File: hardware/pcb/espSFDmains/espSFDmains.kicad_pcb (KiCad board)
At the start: 4 copper layers, 111.8 x 63.5 mm, 40 parts, among them J1 Mains, J10 D1 & D2, J11 D3 & D4, J2 Mains Motor, J3 VDD, J4 D5 & D6, J5 Motor, J8 SFD Bus, J9 SFD Bus, U1 TXS0102DCT, U2 LM2675N-5, U3 WEMOS_D1_mini

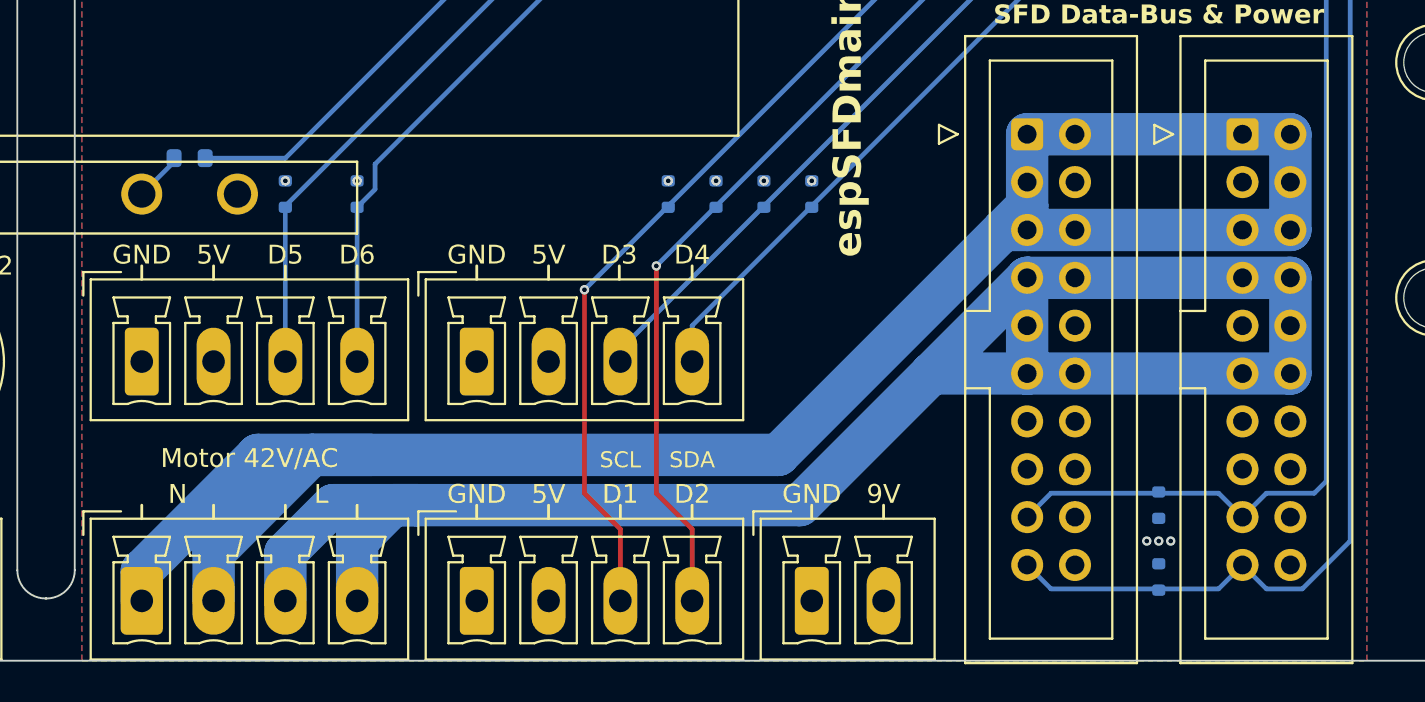
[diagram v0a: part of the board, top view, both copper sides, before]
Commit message: hedfhf
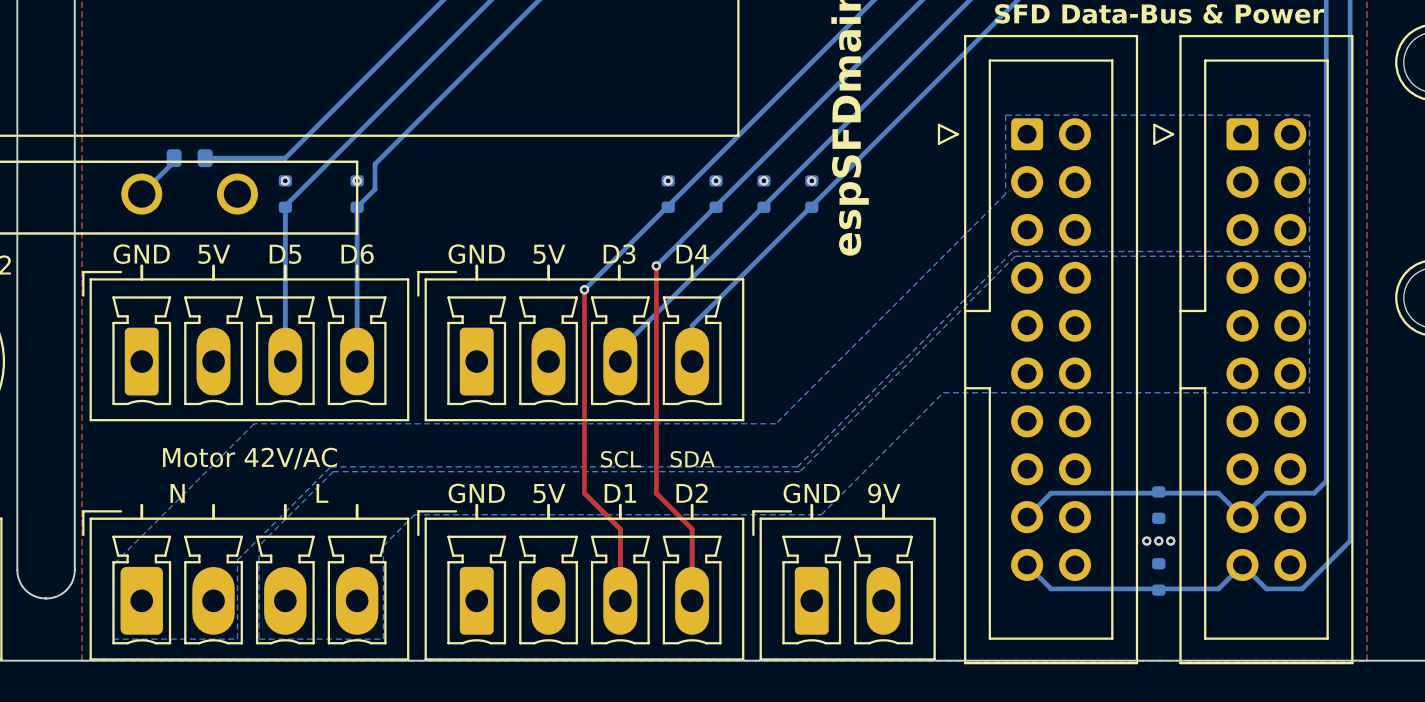
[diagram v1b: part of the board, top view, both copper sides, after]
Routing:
- net Motor N: track 109.0 -> 0.00 mm
- net Motor L: track 100.2 -> 0.00 mm
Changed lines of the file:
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@@
-	)
-	(segment
-		(start 117.155 140.01)
-		(end 122.235 134.93)
-		(width 2.25)
-		(layer "B.Cu")
-		(net 1)
-	)
-	(segment
-		(start 89.85 146.995)
-		(end 88.58 146.995)
-		(width 2.25)
-		(layer "B.Cu")
-		(net 1)
-	)
-	(segment
-		(start 86.675 148.9)
-		(end 86.675 152.075)
-		(width 2.25)
-		(layer "B.Cu")
-		(net 1)
-	)
-	(segment
-		(start 86.675 148.9)
-		(end 86.675 146.995)
-		(width 2.25)
-		(layer "B.Cu")
-		(net 1)
-	)
-	(segment
-		(start 89.85 146.995)
-		(end 86.675 146.995)
-		(width 2.25)
-		(layer "B.Cu")
-		(net 1)
-	)
-	(segment
-		(start 122.235 134.93)
-		(end 122.235 140.01)
-		(width 2.25)
-		(layer "B.Cu")
-		(net 1)
-	)
-	(segment
-		(start 110.17 146.995)
-		(end 117.155 140.01)
-		(width 2.25)
-		(layer "B.Cu")
-		(net 1)
-	)
-	(segment
-		(start 136.205 140.01)
-		(end 122.235 140.01)
-		(width 2.25)
-		(layer "B.Cu")
-		(net 1)
-	)
-	(segment
-		(start 122.235 140.01)
-		(end 117.155 140.01)
-		(width 2.25)
-		(layer "B.Cu")
-		(net 1)
-	)
-	(segment
-		(start 122.235 134.93)
-		(end 136.205 134.93)
-		(width 2.25)
-		(layer "B.Cu")
-		(net 1)
-	)
-	(segment
-		(start 82.865 149.535)
-		(end 82.865 152.075)
-		(width 2.25)
-		(layer "B.Cu")
-		(net 1)
-	)
-	(segment
-		(start 89.85 146.995)
-		(end 110.17 146.995)
-		(width 2.25)
-		(layer "B.Cu")
-		(net 1)
-	)
-	(segment
-		(start 88.58 146.995)
-		(end 86.675 148.9)
-		(width 2.25)
-		(layer "B.Cu")
-		(net 1)
-	)
-	(segment
-		(start 86.675 146.995)
-		(end 85.405 146.995)
-		(width 2.25)
-		(layer "B.Cu")
-		(net 1)
-	)
-	(segment
-		(start 136.205 134.93)
-		(end 136.205 140.01)
-		(width 2.25)
-		(layer "B.Cu")
-		(net 1)
-	)
-	(segment
-		(start 85.405 146.995)
-		(end 82.865 149.535)
-		(width 2.25)
-		(layer "B.Cu")
-		(net 1)
-	)
-	(segment
-		(start 79.055 149.535)
-		(end 84.262 144.328)
-		(width 2.25)
-		(layer "B.Cu")
-		(net 2)
-	)
-	(segment
-		(start 122.235 131.12)
-		(end 122.235 127.31)
-		(width 2.25)
-		(layer "B.Cu")
-		(net 2)
-	)
-	(segment
-		(start 75.245 150.4875)
-		(end 75.245 152.075)
-		(width 2.25)
-		(layer "B.Cu")
-		(net 2)
-	)
-	(segment
-		(start 79.055 152.075)
-		(end 79.055 149.535)
-		(width 2.25)
-		(layer "B.Cu")
-		(net 2)
-	)
-	(segment
-		(start 120.965 132.39)
-		(end 122.235 131.12)
-		(width 2.25)
-		(layer "B.Cu")
-		(net 2)
-	)
-	(segment
-		(start 122.235 127.31)
-		(end 136.205 127.31)
-		(width 2.25)
-		(layer "B.Cu")
-		(net 2)
-	)
-	(segment
-		(start 109.027 144.328)
-		(end 120.965 132.39)
-		(width 2.25)
-		(layer "B.Cu")
-		(net 2)
-	)
-	(segment
-		(start 136.205 132.39)
-		(end 122.235 132.39)
-		(width 2.25)
-		(layer "B.Cu")
-		(net 2)
-	)
-	(segment
-		(start 81.4045 144.328)
-		(end 75.245 150.4875)
-		(width 2.25)
-		(layer "B.Cu")
-		(net 2)
-	)
-	(segment
-		(start 136.205 127.31)
-		(end 136.205 132.39)
-		(width 2.25)
-		(layer "B.Cu")
-		(net 2)
-	)
-	(segment
-		(start 122.235 132.39)
-		(end 122.235 131.12)
-		(width 2.25)
-		(layer "B.Cu")
-		(net 2)
-	)
-	(segment
-		(start 84.262 144.328)
-		(end 109.027 144.328)
-		(width 2.25)
-		(layer "B.Cu")
-		(net 2)
-	)
-	(segment
-		(start 120.965 132.39)
-		(end 122.235 132.39)
-		(width 2.25)
-		(layer "B.Cu")
-		(net 2)
-	)
-	(segment
-		(start 87.437 144.328)
-		(end 81.4045 144.328)
-		(width 2.25)
-		(layer "B.Cu")
-		(net 2)
 	)
 	(segment
@@
 	)
 	(zone
-		(net 2)
-		(net_name "Motor N")
-		(layer "B.Cu")
-		(hatch edge 0.5)
-		(priority 4)
-		(connect_pads yes
-			(clearance 0.2)
-		)
-		(min_thickness 0.25)
-		(filled_areas_thickness no)
-		(fill yes
-			(thermal_gap 0.5)
-			(thermal_bridge_width 0.5)
-		)
-		(polygon
-			(pts
-				(xy 122.235 127.31) (xy 122.235 132.39) (xy 136.205 132.39) (xy 136.205 127.31)
-			)
-		)
-	)
-	(zone
 		(net 10)
 		(net_name "+9V")
@@
 		(layer "B.Cu")
 		(hatch edge 0.5)
-		(priority 4)
-		(connect_pads yes
-			(clearance 0.2)
-		)
-		(min_thickness 0.25)
-		(filled_areas_thickness no)
-		(fill yes
-			(thermal_gap 0.5)
-			(thermal_bridge_width 0.5)
-		)
-		(polygon
-			(pts
-				(xy 122.235 134.93) (xy 136.205 134.93) (xy 136.205 140.01) (xy 117.155 140.01)
-			)
-		)
-	)
-	(zone
-		(net 31)
-		(net_name "+5V")
-		(layer "B.Cu")
-		(hatch edge 0.5)
-		(priority 1)
+		(priority 7)
 		(connect_pads yes
 			(clearance 0.2)
@@
 		(polygon
 			(pts
+				(xy 137.221 133.787) (xy 121.6 133.787) (xy 110.17 145.217) (xy 85.405 145.217) (xy 81.468 149.154)
+				(xy 81.468 154.107) (xy 88.072 154.107) (xy 88.072 149.154) (xy 89.723 147.503) (xy 111.313 147.503)
+				(xy 117.79 141.026) (xy 137.221 141.026)
+			)
+		)
+	)
+	(zone
+		(net 31)
+		(net_name "+5V")
+		(layer "B.Cu")
+		(hatch edge 0.5)
+		(priority 1)
+		(connect_pads yes
+			(clearance 0.2)
+		)
+		(min_thickness 0.25)
+		(filled_areas_thickness no)
+		(fill yes
+			(thermal_gap 0.5)
+			(thermal_bridge_width 0.5)
+			(smoothing fillet)
+			(radius 0.25)
+		)
+		(polygon
+			(pts
 				(xy 87.818 109.911) (xy 84.135 109.911) (xy 80.071 105.847) (xy 80.071 99.751) (xy 83.119 96.83)
 				(xy 83.119 95.687) (xy 83.119 95.052) (xy 86.675 95.052) (xy 86.675 96.068) (xy 84.4525 96.068)
@@
 			)
 		)
+	)
+	(zone
+		(net 2)
+		(net_name "Motor N")
+		(layer "B.Cu")
+		(hatch edge 0.5)
+		(priority 3)
+		(connect_pads yes
+			(clearance 0.2)
+		)
+		(min_thickness 0.25)
+		(filled_areas_thickness no)
+		(fill yes
+			(thermal_gap 0.5)
+			(thermal_bridge_width 0.5)
+			(smoothing fillet)
+			(radius 0.25)
+		)
+		(polygon
+			(pts
+				(xy 137.221 133.533) (xy 137.221 126.294) (xy 121.092 126.294) (xy 121.092 130.485) (xy 108.9 142.677)
+				(xy 81.214 142.677) (xy 73.721 150.17) (xy 73.721 154.107) (xy 80.325 154.107) (xy 80.325 149.916)
+				(xy 85.278 144.963) (xy 110.043 144.963) (xy 121.473 133.533)
+			)
+		)
